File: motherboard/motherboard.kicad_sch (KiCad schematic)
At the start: 21 parts, among them J1 532610471, J2 GSB1C41110SSHR, J3 532610471, J4 532610471, J5 532610471, J6 Conn_01x04_Pin, U1 RP2040, U2 ESP32-C3-WROOM-02U, U3 USBLC6-2SC6, U4 AP2112K-3.3TRG1

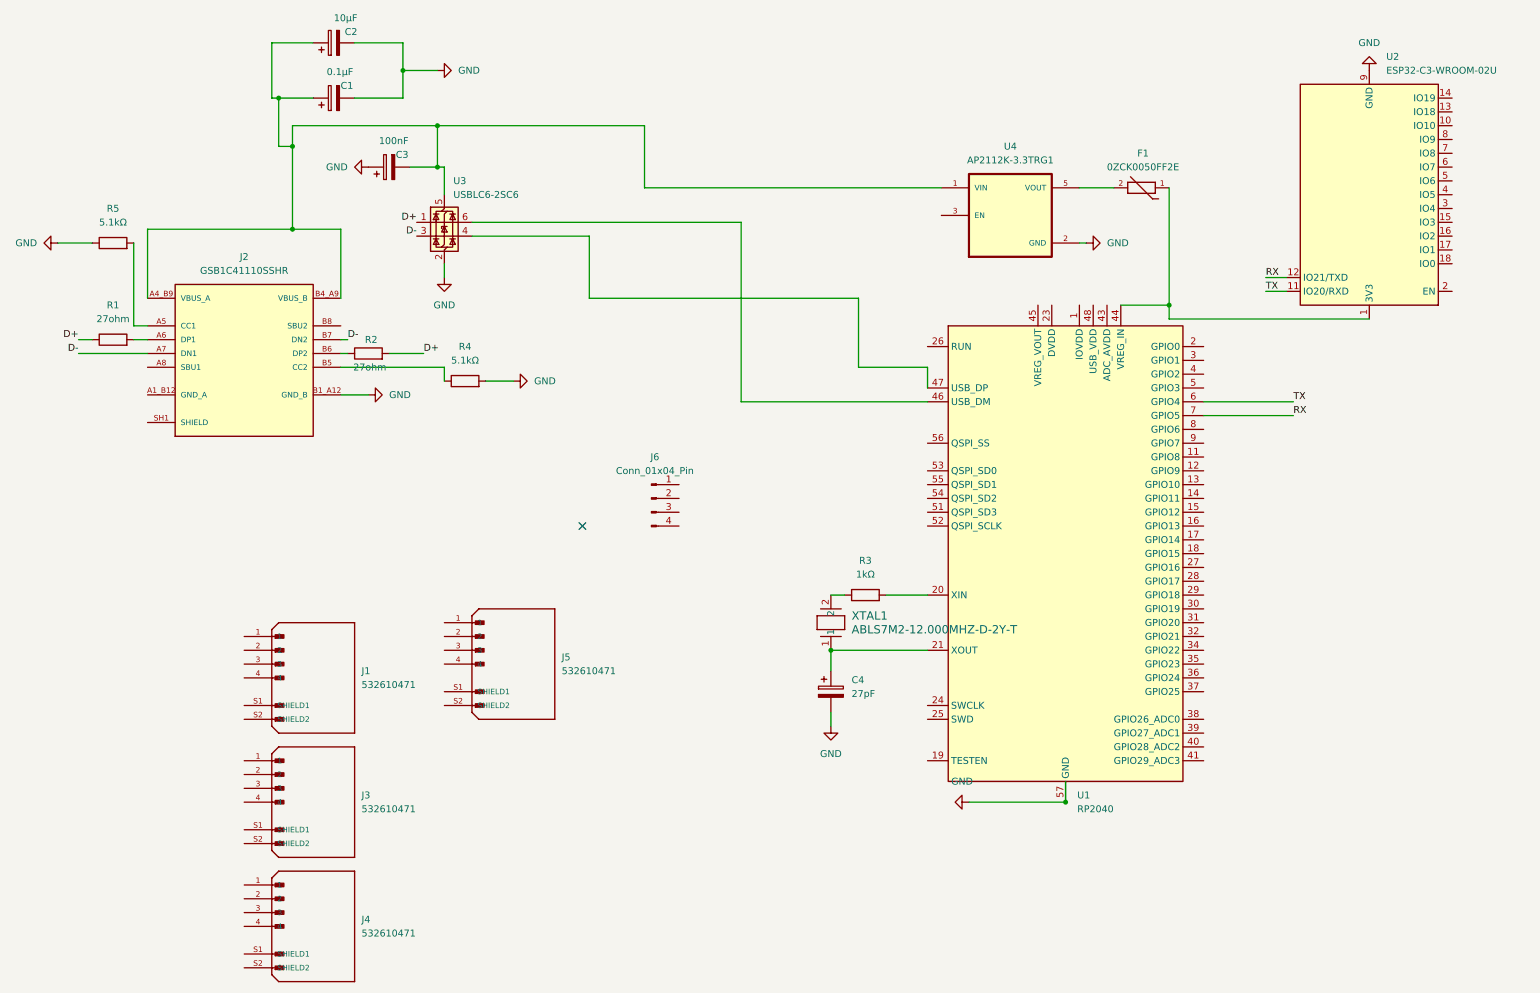
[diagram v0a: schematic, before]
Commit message: fix : change composant
for next day :
- fix molex connector
- fix esp32 routing
- set pcb design
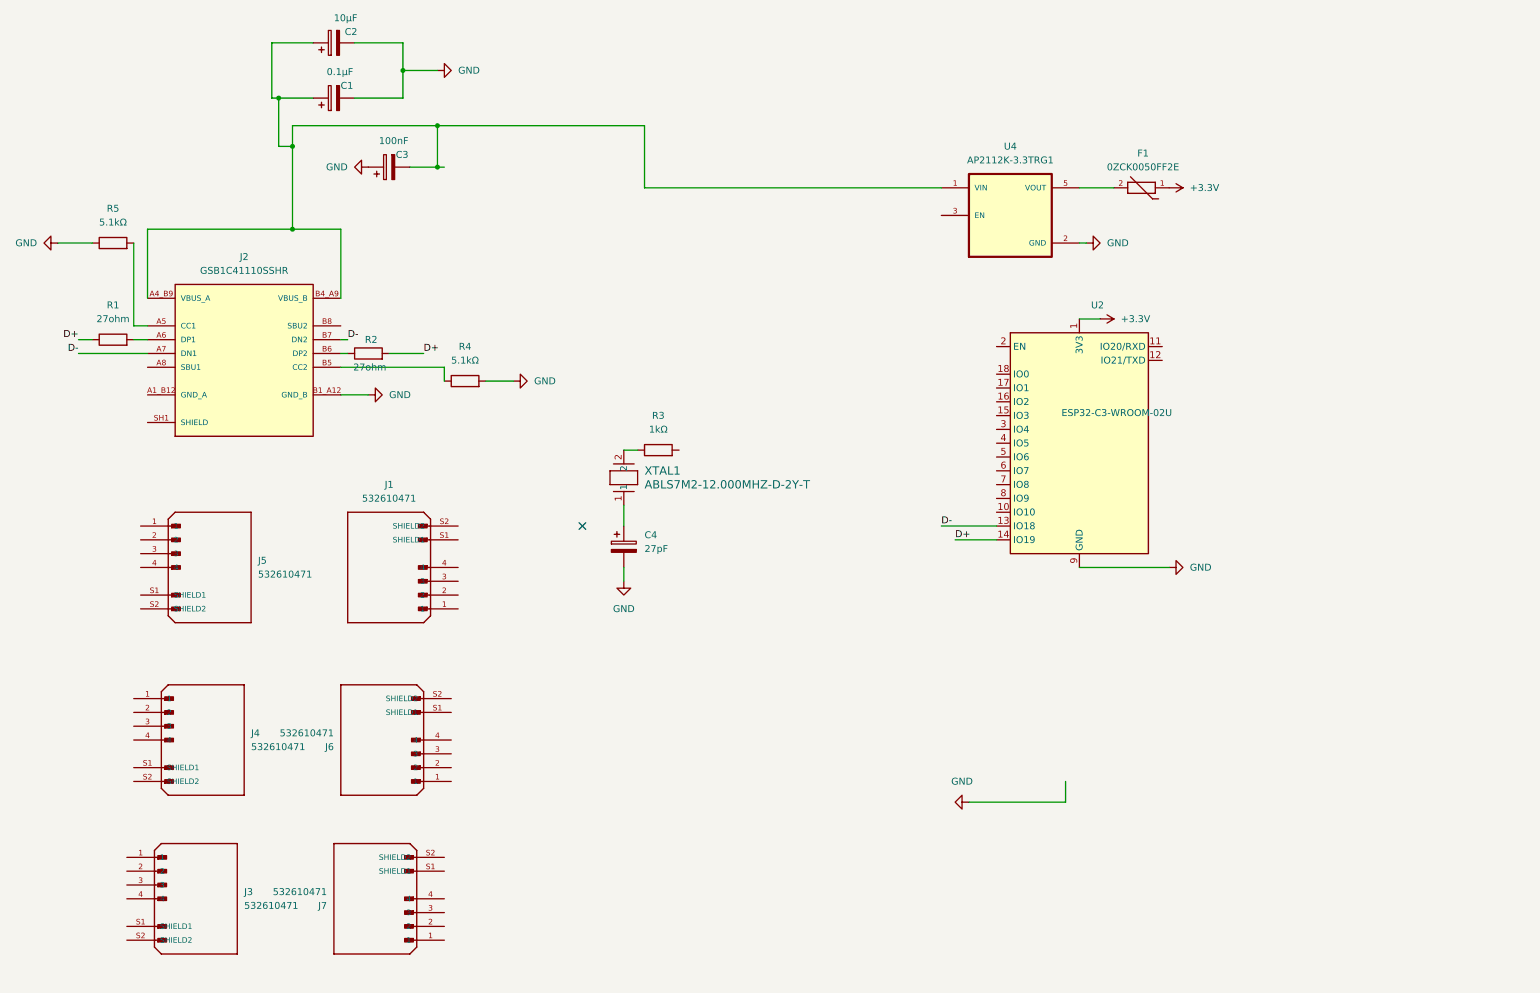
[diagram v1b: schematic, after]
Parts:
- removed J6: Conn_01x04_Pin, Connector_PinHeader_1.00mm:PinHeader_1x04_P1.00mm_Vertical, symbol Connector:Conn_01x04_Pin
- removed U1: RP2040, Package_DFN_QFN:QFN-56-1EP_7x7mm_P0.4mm_EP3.2x3.2mm, symbol MCU_RaspberryPi:RP2040
- removed U3: USBLC6-2SC6, Package_TO_SOT_SMD:SOT-23-6, symbol Power_Protection:USBLC6-2SC6
- added J6, J7: 532610471, Library:MOLEX_532610471, symbol Connector_Header Surface Mount, Right Angle 4 position 0.049{dblquote} (1.25mm)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
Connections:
- net D+: now also U2.14 (IO19)
- net D-: now also U2.13 (IO18)
- net +3.3V: now reaches F1.1, U2.1 (3V3)
- net RX: no longer names the net of U2.12 (IO21/TXD)
- net TX: no longer names the net of U2.11 (IO20/RXD)
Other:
- company: (none) -> Modul X
- title: (none) -> Mother board Modul X
- moved on the sheet: C4, J1, J3, J4, J5, R3, U2, XTAL1
